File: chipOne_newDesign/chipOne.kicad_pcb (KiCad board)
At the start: 4 copper layers, 113 x 113.8 mm, 27 parts

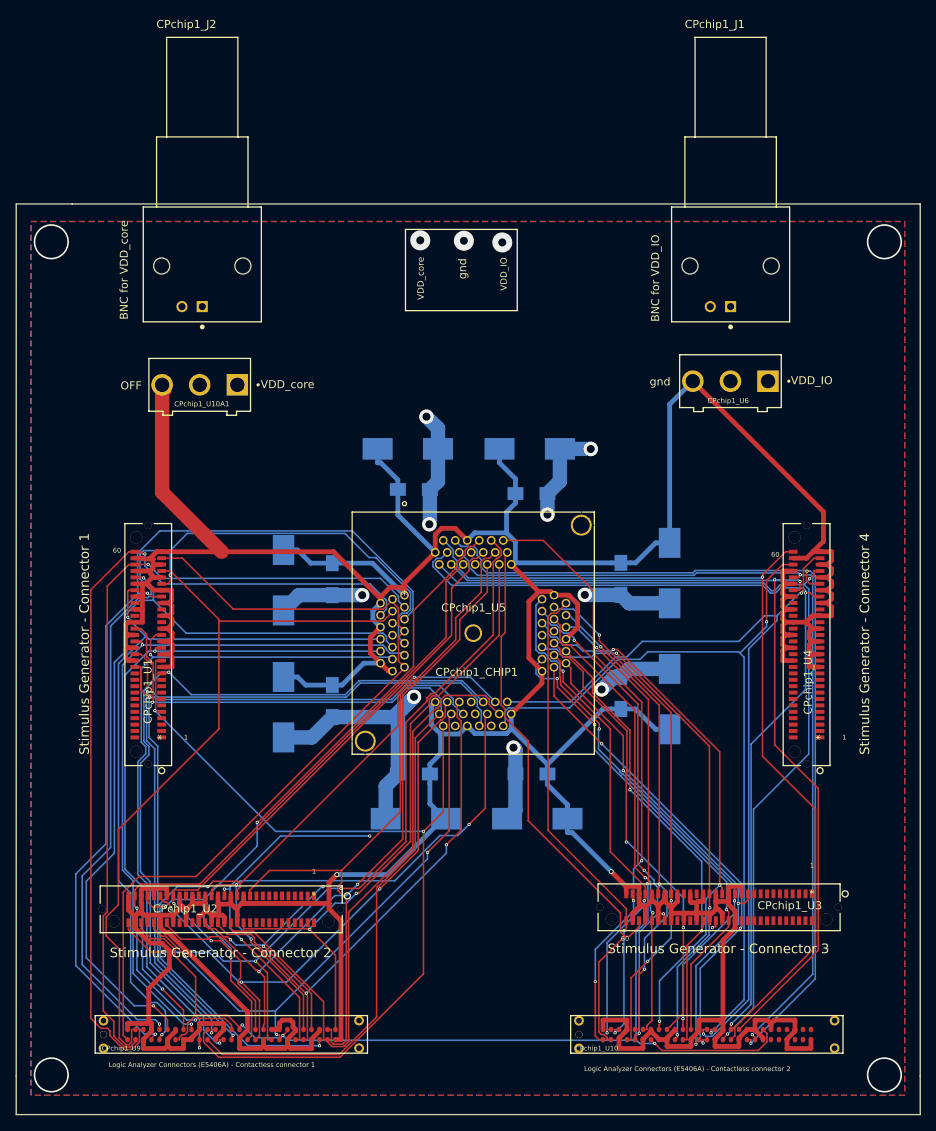
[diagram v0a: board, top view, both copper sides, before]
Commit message: Changes finilised
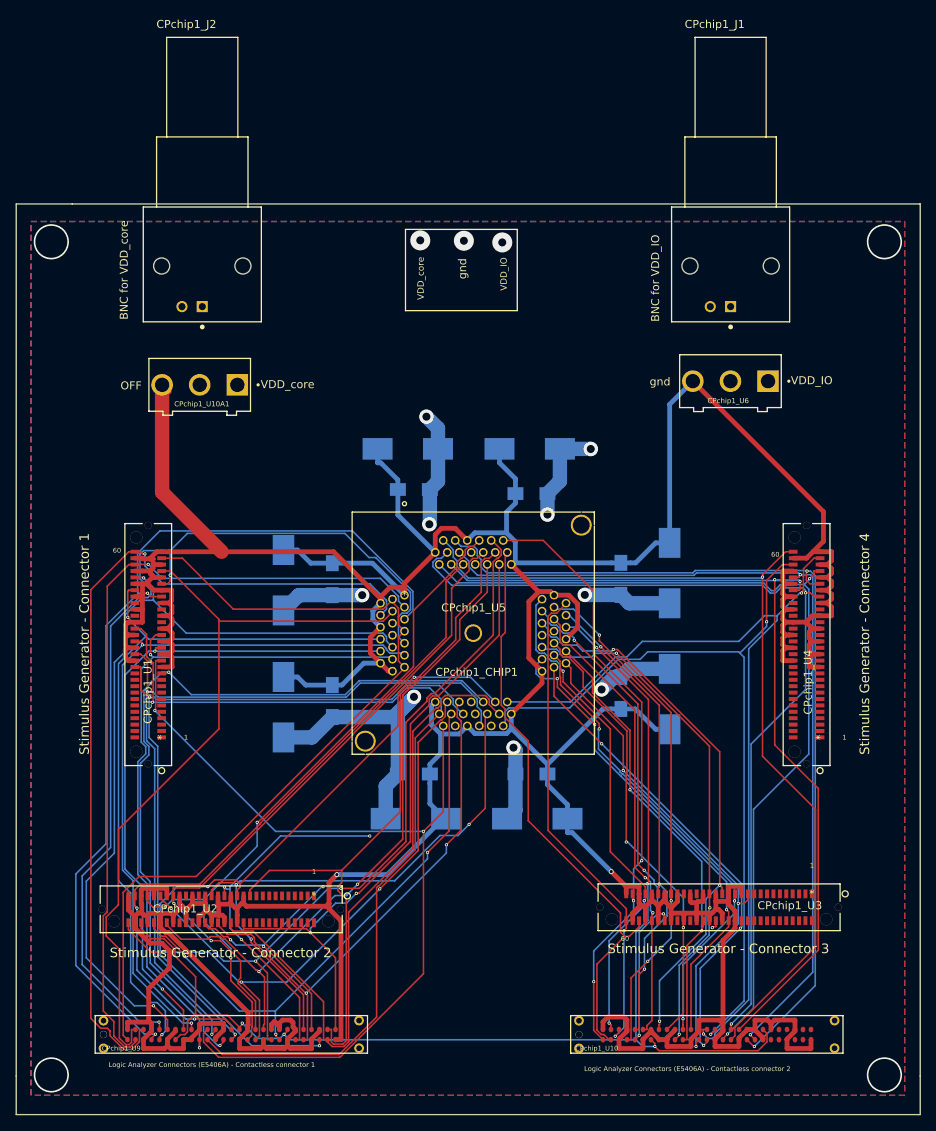
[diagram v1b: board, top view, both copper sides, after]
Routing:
- net VSSQ: track 797.6 -> 799.5 mm
- net B_inData_bi4: track 63.9 -> 62.5 mm
- net I_clk: track 155.1 -> 155.7 mm
- net I_address4: track 113.8 -> 114.4 mm
- net B_outData_bi4: track 61.6 -> 62.2 mm
- net B_inData_bi5: track 60.6 -> 61.1 mm
